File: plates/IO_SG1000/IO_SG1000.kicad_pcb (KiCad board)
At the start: 2 copper layers, 40 x 100 mm, 12 parts, among them J10 NES_Joystick1, J22 PJ320D, J24 Conn_02x10_Odd_Even, J25 Conn_02x20_Odd_Even, U7 SN76489AN

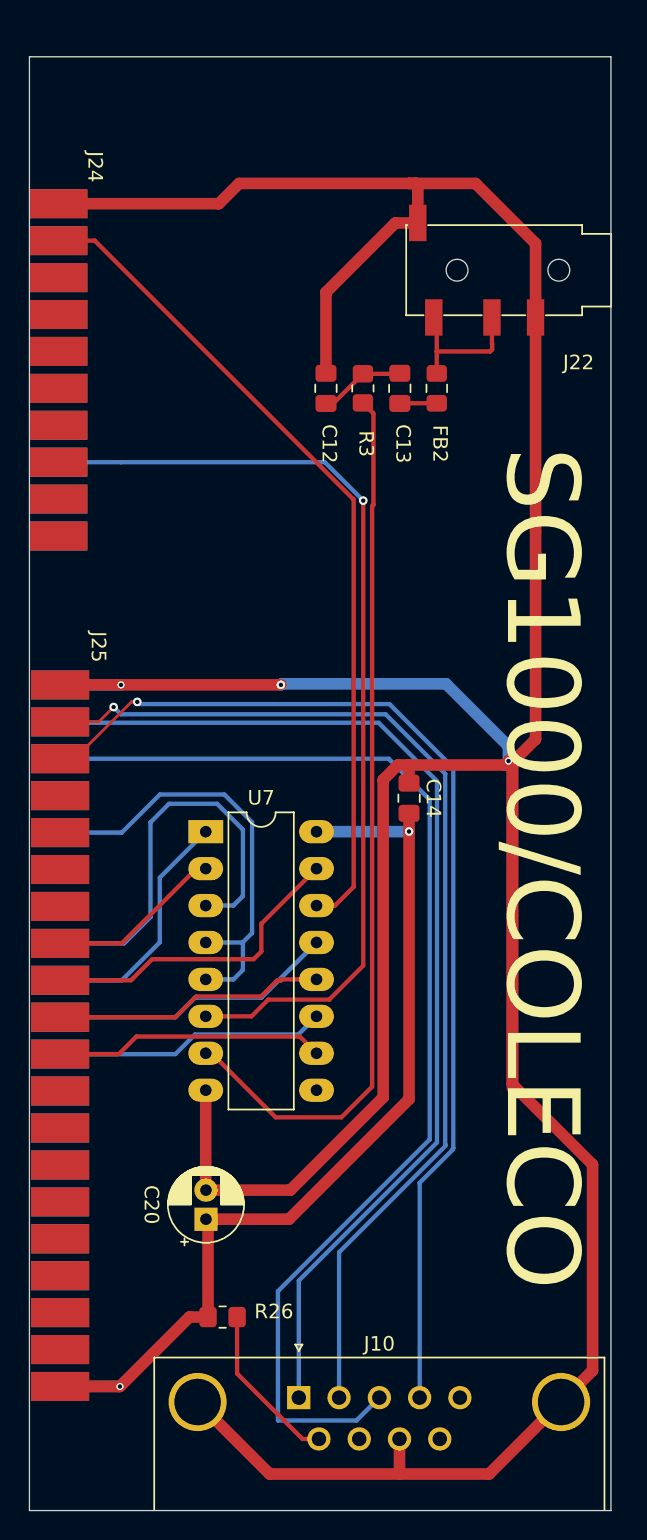
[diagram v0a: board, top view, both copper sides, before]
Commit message: Update IO_SG1000.kicad_pcb
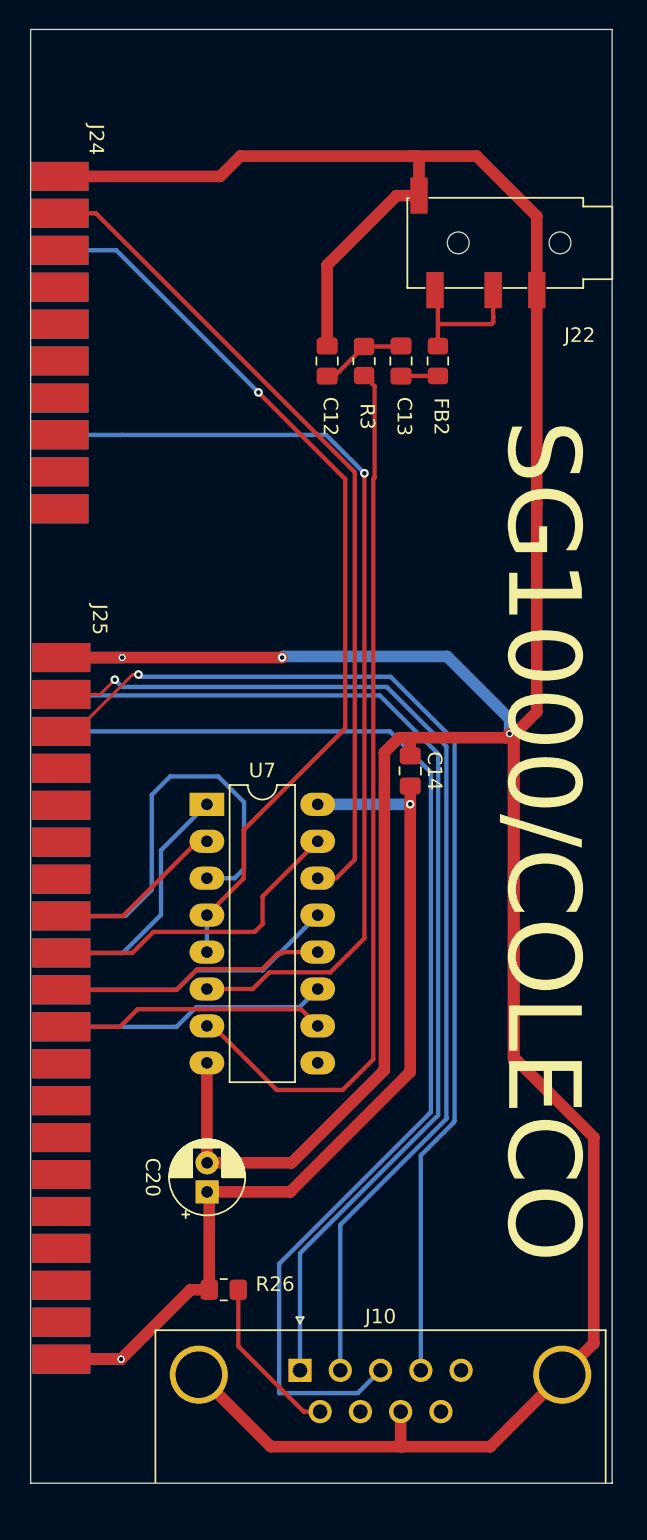
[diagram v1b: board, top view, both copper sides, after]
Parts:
- moved J25 1.88 mm to (126.8, 84.6)
- moved C12 1.88 mm to (145.1, 64.2)
- moved C13 1.88 mm to (150.2, 64.2)
- moved C20 1.88 mm to (136.9, 121.3)
- moved FB2 1.88 mm to (152.7, 64.2)
- moved J24 1.88 mm to (126.7, 51.5)
- moved R3 1.88 mm to (147.7, 64.2)
- moved U7 1.88 mm to (136.8, 94.7)
- moved J22 1.88 mm to (156.4, 56.0)
- moved C14 1.88 mm to (150.8, 92.4)
- moved J10 1.88 mm to (143.2, 133.6)
- moved R26 1.88 mm to (138.0, 128.0)
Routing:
- net (no net): track 1055.3 -> 1087.1 mm, vias 8 -> 9
